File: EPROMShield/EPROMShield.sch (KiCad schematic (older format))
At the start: 17 parts, among them P1 Digital, P10 CONN_01X01, P11 CONN_01X01, P12 CONN_01X01, P13 CONN_01X01, P2 Power, P3 Analog, P4 Analog, P5 PWM, P6 PWM, P7 Communication, P8 CONN_01X01, P9 CONN_01X01

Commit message: Footprints associated
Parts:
- D1, D2: footprint (none) -> LED_SMD:LED_1206_3216Metric_Pad1.42x1.75mm_HandSolder
- R1, R2: footprint (none) -> Resistor_SMD:R_0805_2012Metric_Pad1.20x1.40mm_HandSolder
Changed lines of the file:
@@
 F 0 "D1" V 939 6282 50  0000 R CNN
 F 1 "LED_GN" V 848 6282 50  0000 R CNN
-F 2 "" H 900 6400 50  0001 C CNN
+F 2 "LED_SMD:LED_1206_3216Metric_Pad1.42x1.75mm_HandSolder" H 900 6400 50  0001 C CNN
 F 3 "~" H 900 6400 50  0001 C CNN
 	1    900  6400
@@
 F 0 "R1" H 970 5946 50  0000 L CNN
 F 1 "470" H 970 5855 50  0000 L CNN
-F 2 "" V 830 5900 50  0001 C CNN
+F 2 "Resistor_SMD:R_0805_2012Metric_Pad1.20x1.40mm_HandSolder" V 830 5900 50  0001 C CNN
 F 3 "~" H 900 5900 50  0001 C CNN
 	1    900  5900
@@
 F 0 "D2" V 1589 6282 50  0000 R CNN
 F 1 "LED_RD" V 1498 6282 50  0000 R CNN
-F 2 "" H 1550 6400 50  0001 C CNN
+F 2 "LED_SMD:LED_1206_3216Metric_Pad1.42x1.75mm_HandSolder" H 1550 6400 50  0001 C CNN
 F 3 "~" H 1550 6400 50  0001 C CNN
 	1    1550 6400
@@
 F 0 "R2" H 1620 5946 50  0000 L CNN
 F 1 "470" H 1620 5855 50  0000 L CNN
-F 2 "" V 1480 5900 50  0001 C CNN
+F 2 "Resistor_SMD:R_0805_2012Metric_Pad1.20x1.40mm_HandSolder" V 1480 5900 50  0001 C CNN
 F 3 "~" H 1550 5900 50  0001 C CNN
 	1    1550 5900

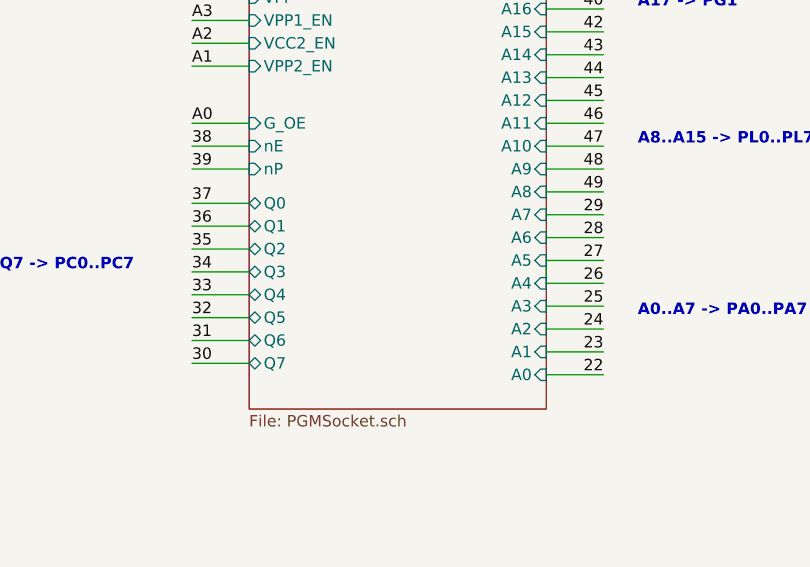
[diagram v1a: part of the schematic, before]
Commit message: First Version routing is done
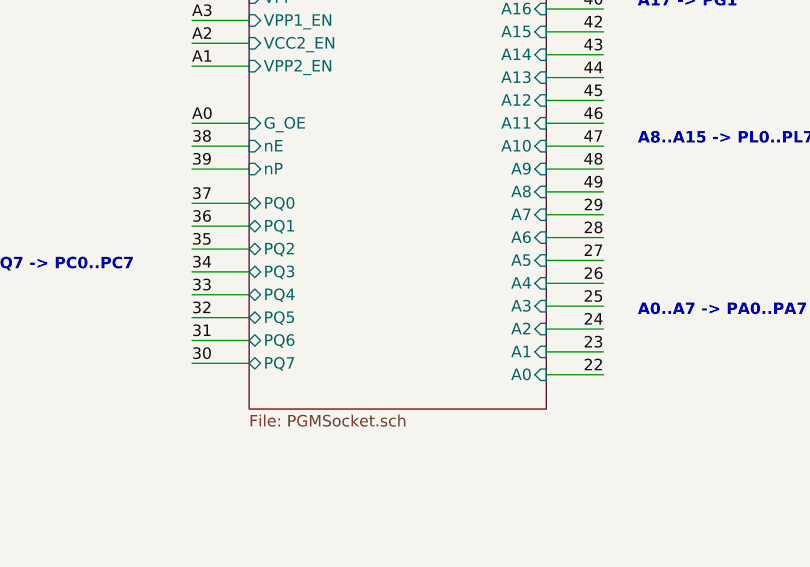
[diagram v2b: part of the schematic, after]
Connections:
- net 26: no longer P1.30 (Pin_30)
- new net 27: P1.30 (Pin_30)
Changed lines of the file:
@@
 Wire Wire Line
 	4900 1700 5050 1700
-$Sheet
-S 3700 3000 1300 2000
-U 6126FB03
-F0 "PGMSocket" 50
-F1 "PGMSocket.sch" 50
-F2 "VCC" I L 3700 3100 50
-F3 "VPP" I L 3700 3200 50
-F4 "VPP1_EN" I L 3700 3300 50
-F5 "VCC2_EN" I L 3700 3400 50
-F6 "A17" I R 5000 3150 50
-F7 "VPP2_EN" I L 3700 3500 50
-F8 "G_OE" I L 3700 3750 50
-F9 "A16" I R 5000 3250 50
-F10 "A15" I R 5000 3350 50
-F11 "A12" I R 5000 3650 50
-F12 "A7" I R 5000 4150 50
-F13 "A6" I R 5000 4250 50
-F14 "A5" I R 5000 4350 50
-F15 "A4" I R 5000 4450 50
-F16 "A3" I R 5000 4550 50
-F17 "A2" I R 5000 4650 50
-F18 "A1" I R 5000 4750 50
-F19 "A0" I R 5000 4850 50
-F20 "nE" I L 3700 3850 50
-F21 "A11" I R 5000 3750 50
-F22 "A9" I R 5000 3950 50
-F23 "A8" I R 5000 4050 50
-F24 "A13" I R 5000 3550 50
-F25 "A14" I R 5000 3450 50
-F26 "nP" I L 3700 3950 50
-F27 "Q0" B L 3700 4100 50
-F28 "Q1" B L 3700 4200 50
-F29 "Q2" B L 3700 4300 50
-F30 "Q3" B L 3700 4400 50
-F31 "Q4" B L 3700 4500 50
-F32 "Q5" B L 3700 4600 50
-F33 "Q6" B L 3700 4700 50
-F34 "Q7" B L 3700 4800 50
-F35 "A10" I R 5000 3850 50
-$EndSheet
 Wire Wire Line
 	3700 4100 3450 4100
@@
 	5000 4550 5250 4550
 Wire Wire Line
-	5000 4450 5000 4350
-Wire Wire Line
-	5000 4450 5250 4450
-Wire Wire Line
-	5000 4350 5250 4350
-Wire Wire Line
 	5000 4250 5250 4250
 Wire Wire Line
@@
 Text Label 5250 4550 2    50   ~ 0
 25
-Text Label 5250 4450 2    50   ~ 0
-26
-Text Label 5250 4350 2    50   ~ 0
-27
 Text Label 5250 4250 2    50   ~ 0
 28
@@
 	1    0    0    -1
 $EndComp
-Wire Wire Line
-	900  5550 900  5750
 $Comp
 L Device:LED D?
@@
 Text Label 3600 1700 0    50   ~ 0
 +5V
+Wire Wire Line
+	5000 4350 5250 4350
+Wire Wire Line
+	5000 4450 5250 4450
+$Sheet
+S 3700 3000 1300 2000
+U 6126FB03
+F0 "PGMSocket" 50
+F1 "PGMSocket.sch" 50
+F2 "VCC" I L 3700 3100 50
+F3 "VPP" I L 3700 3200 50
+F4 "VPP1_EN" I L 3700 3300 50
+F5 "VCC2_EN" I L 3700 3400 50
+F6 "A17" I R 5000 3150 50
+F7 "VPP2_EN" I L 3700 3500 50
+F8 "G_OE" I L 3700 3750 50
+F9 "A16" I R 5000 3250 50
+F10 "A15" I R 5000 3350 50
+F11 "A12" I R 5000 3650 50
+F12 "A7" I R 5000 4150 50
+F13 "A6" I R 5000 4250 50
+F14 "A5" I R 5000 4350 50
+F15 "A4" I R 5000 4450 50
+F16 "A3" I R 5000 4550 50
+F17 "A2" I R 5000 4650 50
+F18 "A1" I R 5000 4750 50
+F19 "A0" I R 5000 4850 50
+F20 "nE" I L 3700 3850 50
+F21 "A11" I R 5000 3750 50
+F22 "A9" I R 5000 3950 50
+F23 "A8" I R 5000 4050 50
+F24 "A13" I R 5000 3550 50
+F25 "A14" I R 5000 3450 50
+F26 "nP" I L 3700 3950 50
+F27 "PQ0" B L 3700 4100 50
+F28 "PQ1" B L 3700 4200 50
+F29 "PQ2" B L 3700 4300 50
+F30 "PQ3" B L 3700 4400 50
+F31 "PQ4" B L 3700 4500 50
+F32 "PQ5" B L 3700 4600 50
+F33 "PQ6" B L 3700 4700 50
+F34 "PQ7" B L 3700 4800 50
+F35 "A10" I R 5000 3850 50
+$EndSheet
+Text Label 5250 4350 2    50   ~ 0
+27
+Text Label 5250 4450 2    50   ~ 0
+26
+Wire Wire Line
+	900  5550 900  5750
 $EndSCHEMATC
